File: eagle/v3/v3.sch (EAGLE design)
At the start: 51 parts, among them IC1 MEGA8-AI

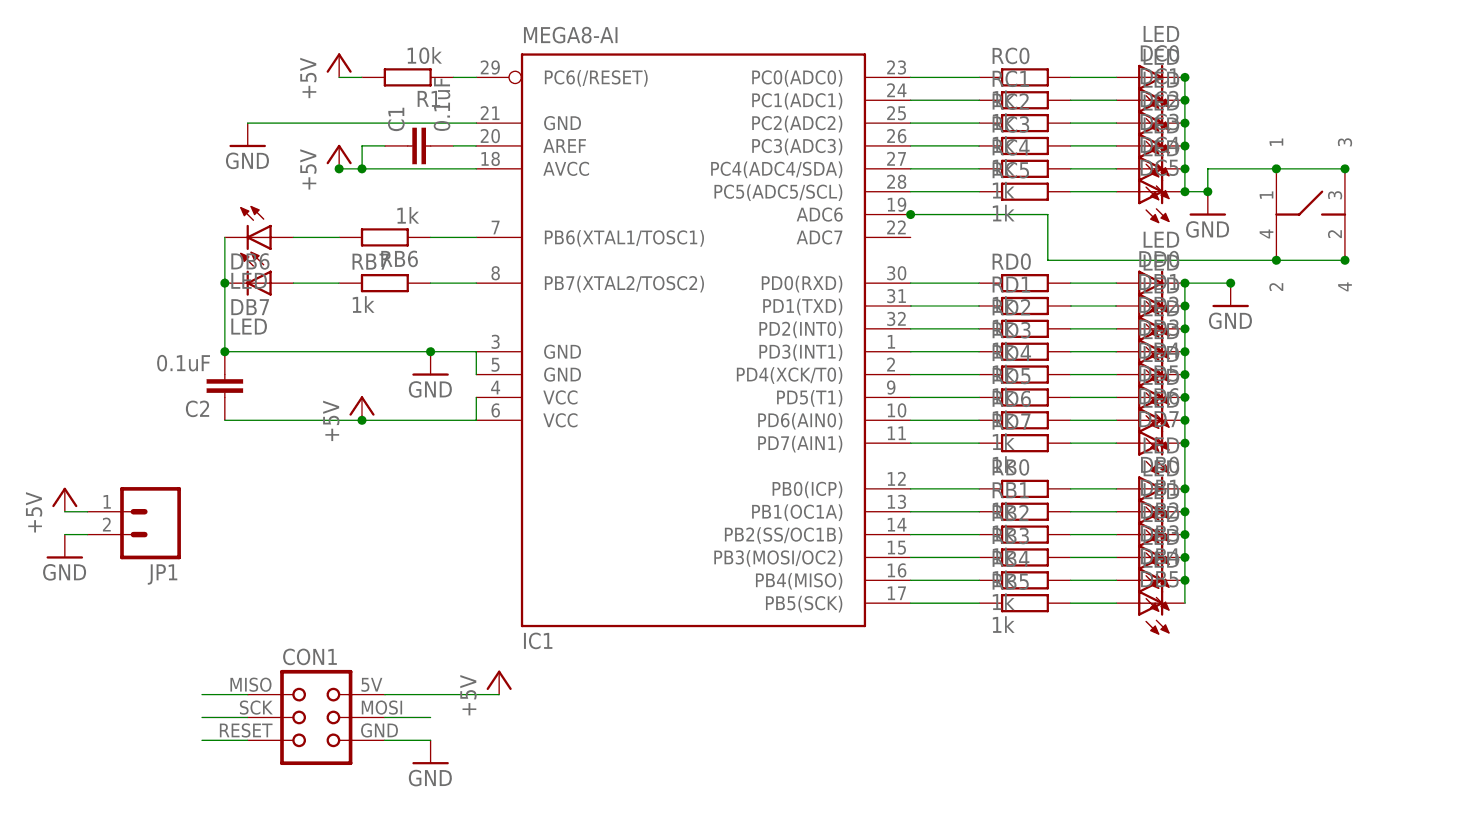
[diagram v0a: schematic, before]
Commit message: Update smiley
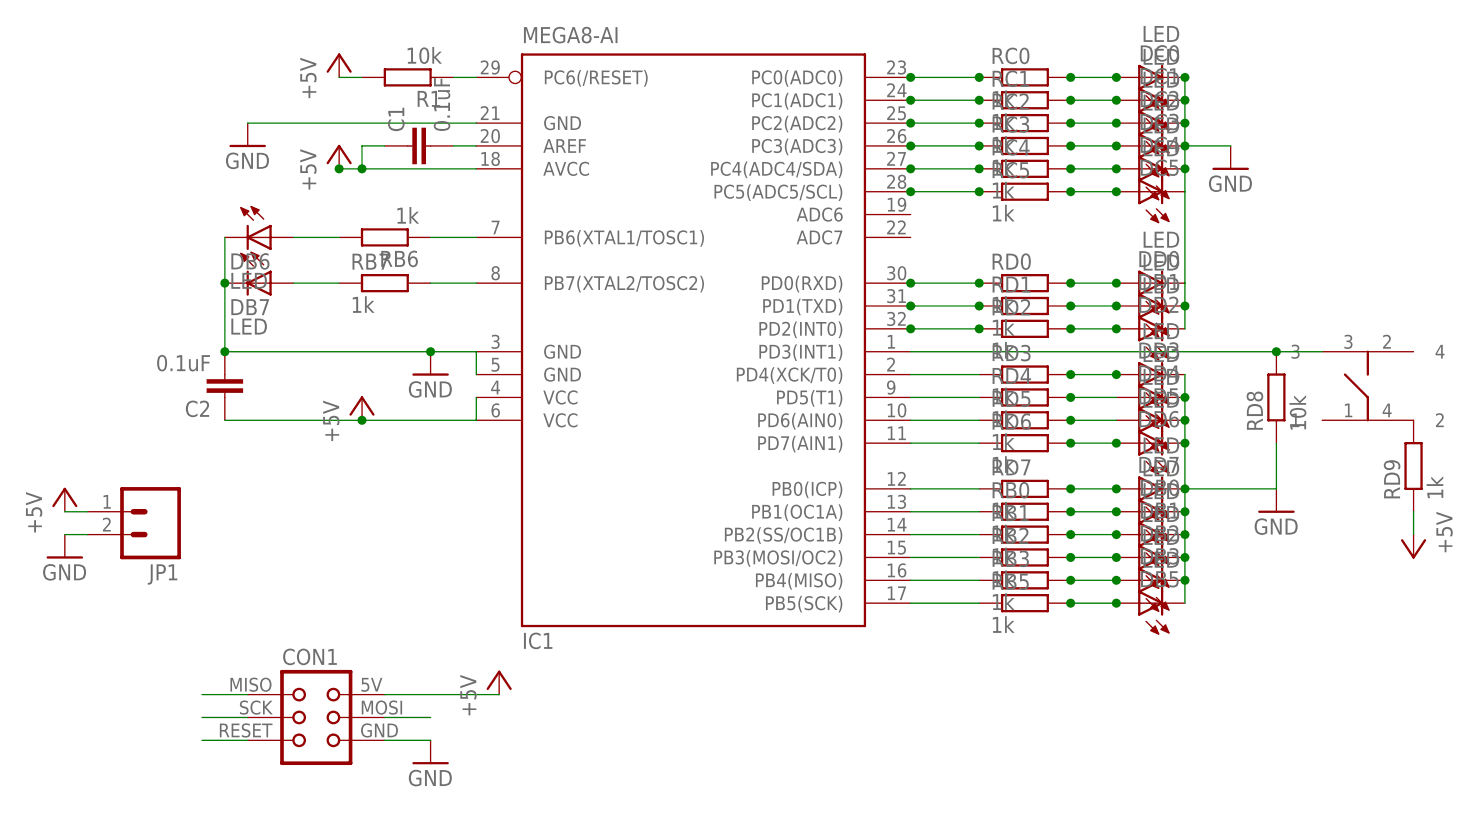
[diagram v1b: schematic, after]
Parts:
- removed DB4: LED, florian:LED
- removed RB4: 1k, resistor:R-EU_R0402
- added RD8: 10k, resistor:R-EU_R0402
- added RD9: 1k, resistor:R-EU_R0402
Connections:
- new net N$45: IC1.PD3(INT1), RD8.2
- net +5V: now also RD9.1
- net GND: now also RD8.1; no longer DB4.C
- net MISO: no longer IC1.PB4(MISO), RB4.1
- net MOSI: no longer IC1.PB3(MOSI/OC2), RB3.1
- net N$11: now also IC1.PB5(SCK), RB5.1; no longer IC1.PD3(INT1), RD3.1
- net N$13: now also IC1.PB4(MISO), RB3.1; no longer IC1.PD5(T1), RD5.1
- net N$14: now also IC1.PB3(MOSI/OC2), RB2.1; no longer IC1.PD4(XCK/T0), RD4.1
- net N$15: now also IC1.PB2(SS/OC1B), RB1.1; no longer IC1.PD6(AIN0), RD6.1
- net N$16: now also IC1.PB1(OC1A), RB0.1; no longer IC1.PD7(AIN1), RD7.1
- net N$17: now also RD7.1; no longer RB0.1
- net N$18: now also IC1.PD7(AIN1), RD6.1; no longer IC1.PB1(OC1A), RB1.1
- net N$19: now also IC1.PD6(AIN0), RD5.1; no longer IC1.PB2(SS/OC1B), RB2.1
- net N$20: now also IC1.PD5(T1), RD4.1; no longer IC1.ADC6
- net N$43: now also IC1.PD4(XCK/T0), RD3.1; no longer DB4.A, RB4.2
- net SCK: no longer IC1.PB5(SCK), RB5.1
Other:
- moved on the sheet: DB0, DB1, DB2, DB3, DD3, DD4, DD5, DD6, DD7, RB0, RB1, RB2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
